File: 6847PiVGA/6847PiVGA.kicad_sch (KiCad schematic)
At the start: 38 parts, among them J1 DB15_Female_HighDensity, U1 MC6847, U2 AD724JRZ, U3 Pico, U4 AD813, Y1 4.433620MHz

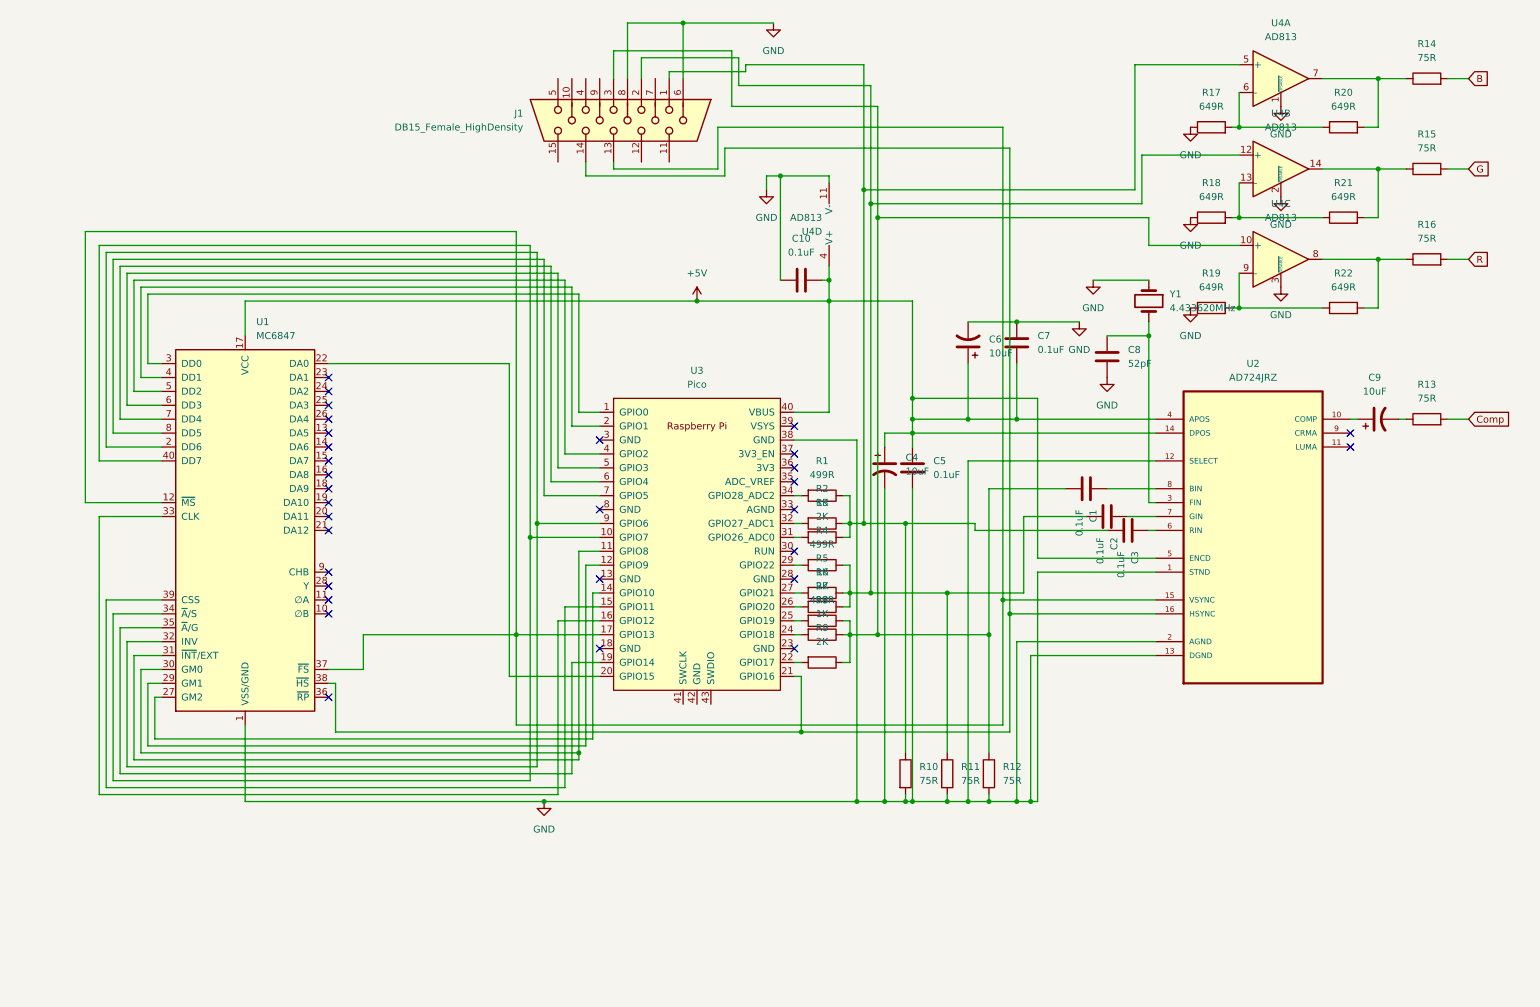
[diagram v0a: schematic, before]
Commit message: board refresh
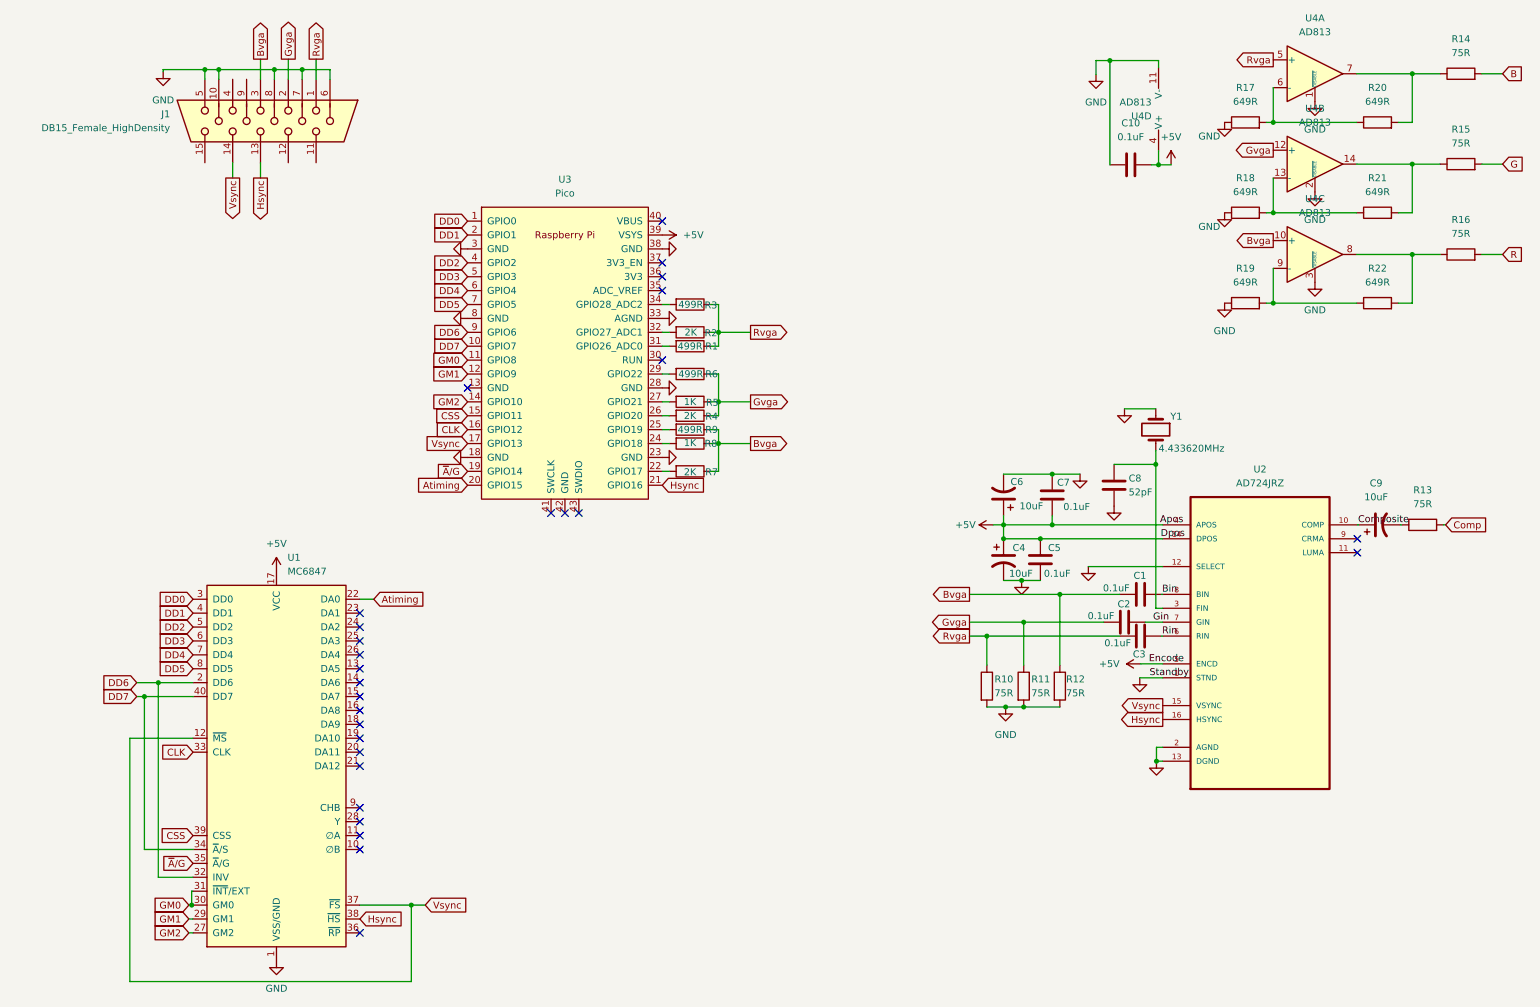
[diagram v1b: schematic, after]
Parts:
- C1, C10, C2, C3, C4, C5, C6, C7, C8, C9: footprint Capacitor_SMD:C_0603_1608Metric -> Capacitor_SMD:C_0805_2012Metric
- R1, R10, R11, R12, R13, R14, R15, R16, R17, R18, R19, R20, R21, R22, R5, R8: footprint Resistor_SMD:R_0603_1608Metric -> Resistor_SMD:R_0805_2012Metric
- R2: value 1K -> 2K; footprint Resistor_SMD:R_0603_1608Metric -> Resistor_SMD:R_0805_2012Metric
- R3, R6, R9: value 2K -> 499R; footprint Resistor_SMD:R_0603_1608Metric -> Resistor_SMD:R_0805_2012Metric
- R4, R7: value 499R -> 2K; footprint Resistor_SMD:R_0603_1608Metric -> Resistor_SMD:R_0805_2012Metric
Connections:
- net +5V: now also U3.39 (VSYS); no longer U3.40 (VBUS)
- net GND: now also J1.10, J1.5, J1.7, U3.18 (GND), U3.23 (GND), U3.28 (GND), U3.3 (GND), U3.33 (AGND), U3.8 (GND)
- net Vsync: now reaches U1.12 (~{MS}), U1.37 (~{FS}), U2.15 (VSYNC), U3.17 (GPIO13)
- net Vsync: now also J1.14; no longer J1.13
- net DD6: now reaches U1.2 (DD6), U1.32 (INV), U3.9 (GPIO6)
- net Atiming: now reaches U1.22 (DA0), U3.20 (GPIO15)
- net GM2: now reaches U1.27 (GM2), U3.14 (GPIO10)
- net GM1: now reaches U1.29 (GM1), U3.12 (GPIO9)
- net DD0: now reaches U1.3 (DD0), U3.1 (GPIO0)
- net GM0: now reaches U1.30 (GM0), U1.31 (~{INT}/EXT), U3.11 (GPIO8)
- net CLK: now reaches U1.33 (CLK), U3.16 (GPIO12)
- net DD7: now reaches U1.34 (~{A}/S), U1.40 (DD7), U3.10 (GPIO7)
- net ~{A}/G: now reaches U1.35 (~{A}/G), U3.19 (GPIO14)
- net Hsync: now reaches U1.38 (~{HS}), U2.16 (HSYNC), U3.21 (GPIO16)
- net Hsync: now also J1.13; no longer J1.14
- net CSS: now reaches U1.39 (CSS), U3.15 (GPIO11)
- net DD1: now reaches U1.4 (DD1), U3.2 (GPIO1)
- net DD2: now reaches U1.5 (DD2), U3.4 (GPIO2)
- net DD3: now reaches U1.6 (DD3), U3.5 (GPIO3)
- net DD4: now reaches U1.7 (DD4), U3.6 (GPIO4)
- net DD5: now reaches U1.8 (DD5), U3.7 (GPIO5)
- net Gvga: now reaches C2.2, J1.2, R11.1, R4.1, R5.1, R6.1, U4.12 (+)
- net at R6.2: now also U3.29 (GPIO22); no longer U3.26 (GPIO20)
- net Bvga: now reaches C1.2, J1.3, R12.1, R7.1, R8.1, R9.1, U4.10 (+)
- net at R7.2: now also U3.22 (GPIO17); no longer U3.25 (GPIO19)
- net Composite: now reaches C9.1, U2.10 (COMP)
- net Rin: now reaches C3.1, U2.6 (RIN)
- net Gin: now reaches C2.1, U2.7 (GIN)
- net Bin: now reaches C1.1, U2.8 (BIN)
- net Rvga: now reaches C3.2, J1.1, R1.1, R10.1, R2.1, R3.1, U4.5 (+)
- net at R3.2: now also U3.34 (GPIO28_ADC2); no longer U3.31 (GPIO26_ADC0)
- net at R9.2: now also U3.25 (GPIO19); no longer U3.22 (GPIO17)
- net at R4.2: now also U3.26 (GPIO20); no longer U3.29 (GPIO22)
- net at R1.2: now also U3.31 (GPIO26_ADC0); no longer U3.34 (GPIO28_ADC2)
- no-connect marks 31 -> 28
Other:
- moved on the sheet: C1, C10, C2, C3, C4, C5, C6, C7, C8, C9, J1, R1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
